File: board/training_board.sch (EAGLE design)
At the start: 24 parts, among them J1 MAIN_PWR, J2 1X2-3.5MM, J3 1X2-3.5MM, Q1 ARDUINOR3-NOIOREF-NOTEXT, SW2 PTS645, U1 ZXBM5210-S-13, U2 ZXBM5210-S-13

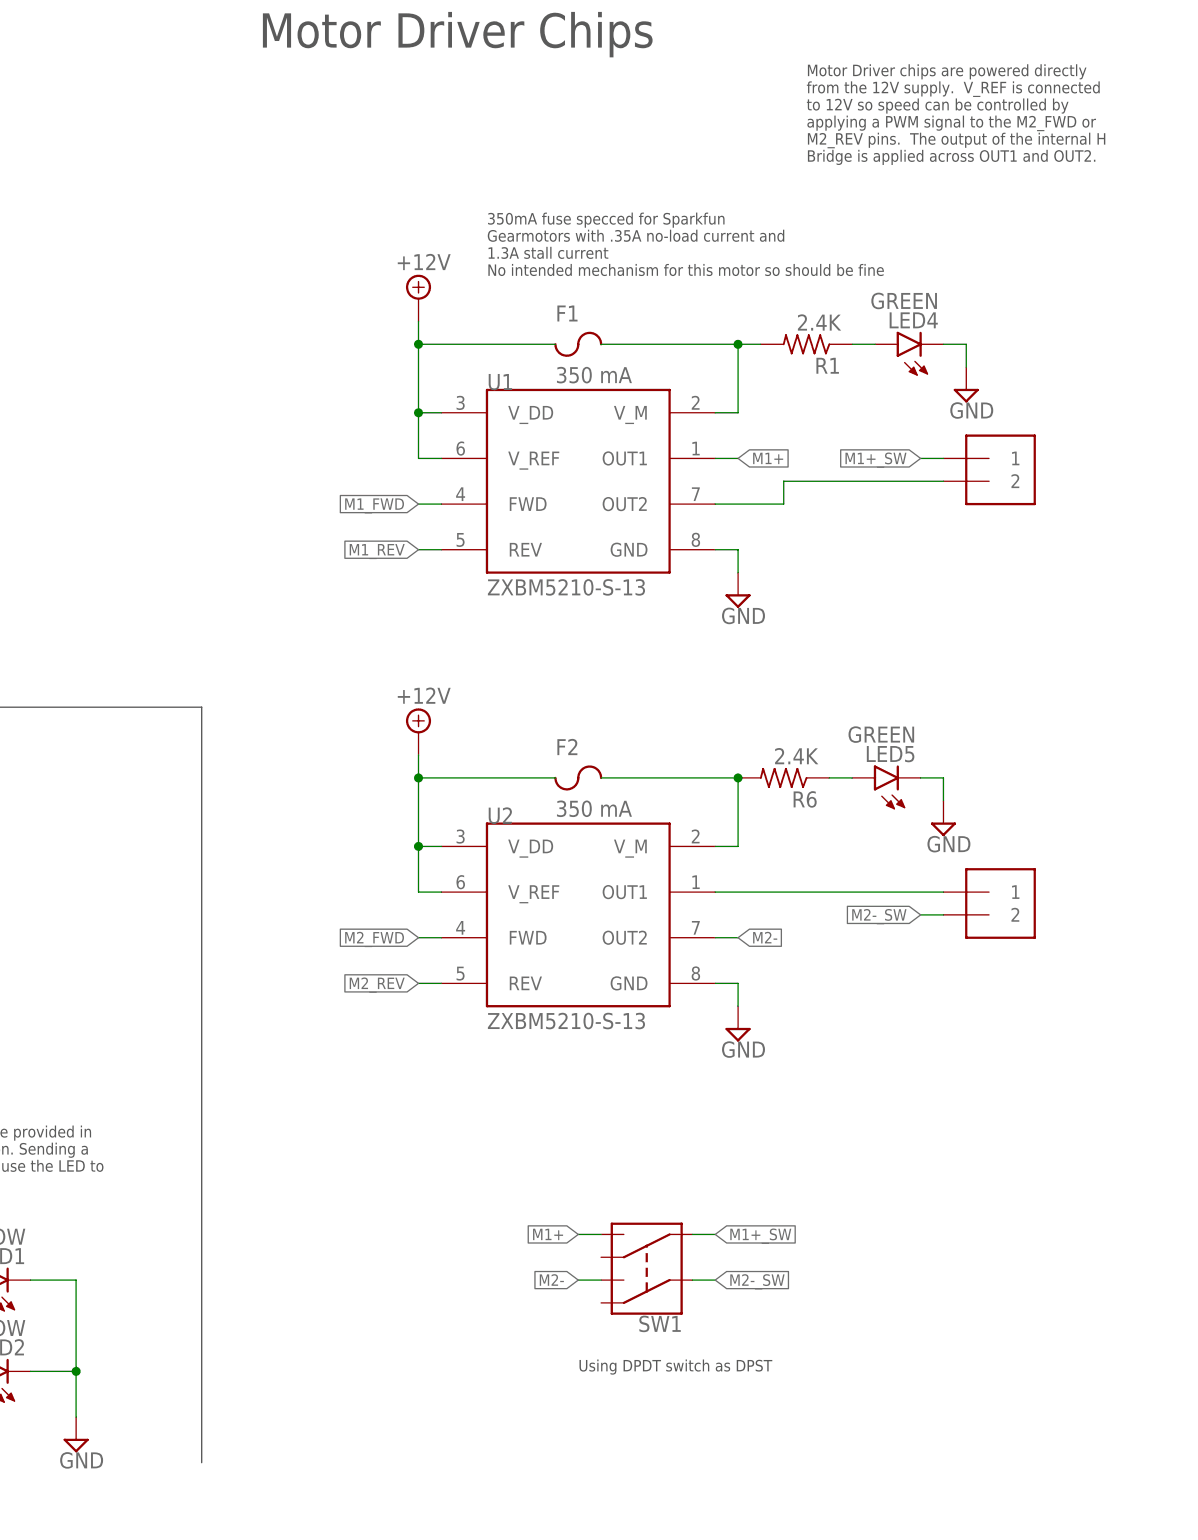
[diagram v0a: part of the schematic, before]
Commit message: Removed 1 motor driver chip from training board
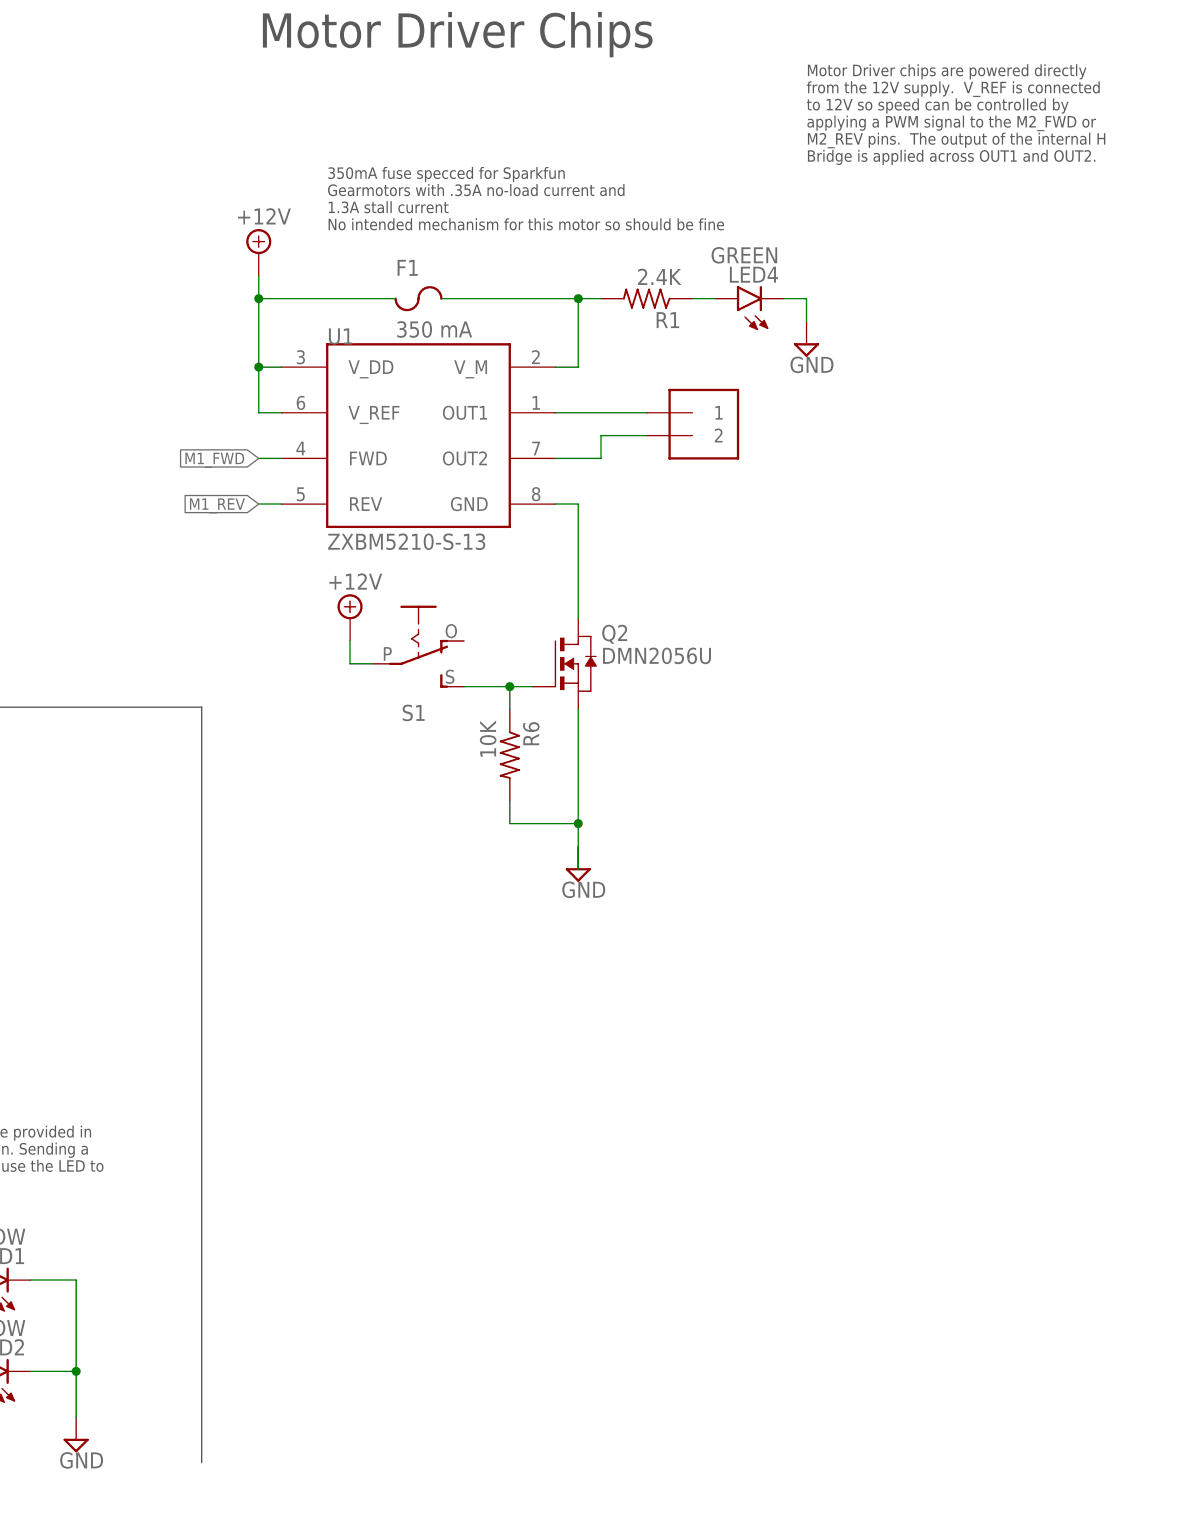
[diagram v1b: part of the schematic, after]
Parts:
- removed F2: 350 mA, RoboJackets-Fuses:CHIP_FUSE1812
- removed J2: 1X2-3.5MM, adafruit:1X2-3.5MM
- removed LED5: GREEN, led:LEDCHIP-LED0603
- removed SW1: (no value), RoboJackets-Switches:400AWMDP1R1M2
- removed U2: ZXBM5210-S-13, RoboJackets-ICs:ZXBM5210-S-13
- added Q2: DMN2056U, RoboJackets-Discrete:NMOSSOT-23-3
- added S1: (no value), adafruit:EG1218S
- R6: value 2.4K -> 10K
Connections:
- removed net M1+: SW1.NO2, U1.OUT1
- removed net M2-: SW1.NO1, U2.OUT2
- removed net M2-_SW: J2.2, SW1.C1
- removed net N$7: F2.2, R6.2, U2.V_M
- removed net N$9: LED5.A, R6.1
- new net N$5: Q2.G, R6.1, S1.S
- net +12V: now also S1.P; no longer F2.1, U2.V_DD, U2.V_REF
- net GND: now also Q2.S, R6.2; no longer LED5.C, U1.GND, U2.GND
- net M1+_SW: now also U1.OUT1; no longer SW1.C2
- net M2_FWD: no longer U2.FWD
- net M2_REV: no longer U2.REV
- net N$3: now also Q2.D, U1.GND; no longer J2.1, U2.OUT1
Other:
- note removed: "Using DPDT switch as DPST"
- moved on the sheet: F1, LED4, R1, R6, U1
